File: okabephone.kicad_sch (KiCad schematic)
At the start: 41 parts, among them J1 Micro_SD_Card_Det1, J2 USB_C_Receptacle_USB2.0_16P, M1 Motor_DC, Q1 AO3400A, SW1 SW_Push, SW10 SW_Push, SW11 SW_Push, SW12 SW_Push, SW13 SW_Push, SW14 SW_Push, SW15 SW_Push, SW16 SW_Push, SW17 SW_Push, SW18 SW_Push, SW19 SW_Push, SW2 SW_Push, SW3 SW_Push, SW4 SW_Push, SW5 SW_Push, SW6 SW_Push, SW7 SW_Push, SW8 SW_Push, SW9 SW_Push, U1 MCP23017_ML, U2 ESP32-S3-WROOM-1, U4 SIM7080G, U5 LD1117S33TR_SOT223

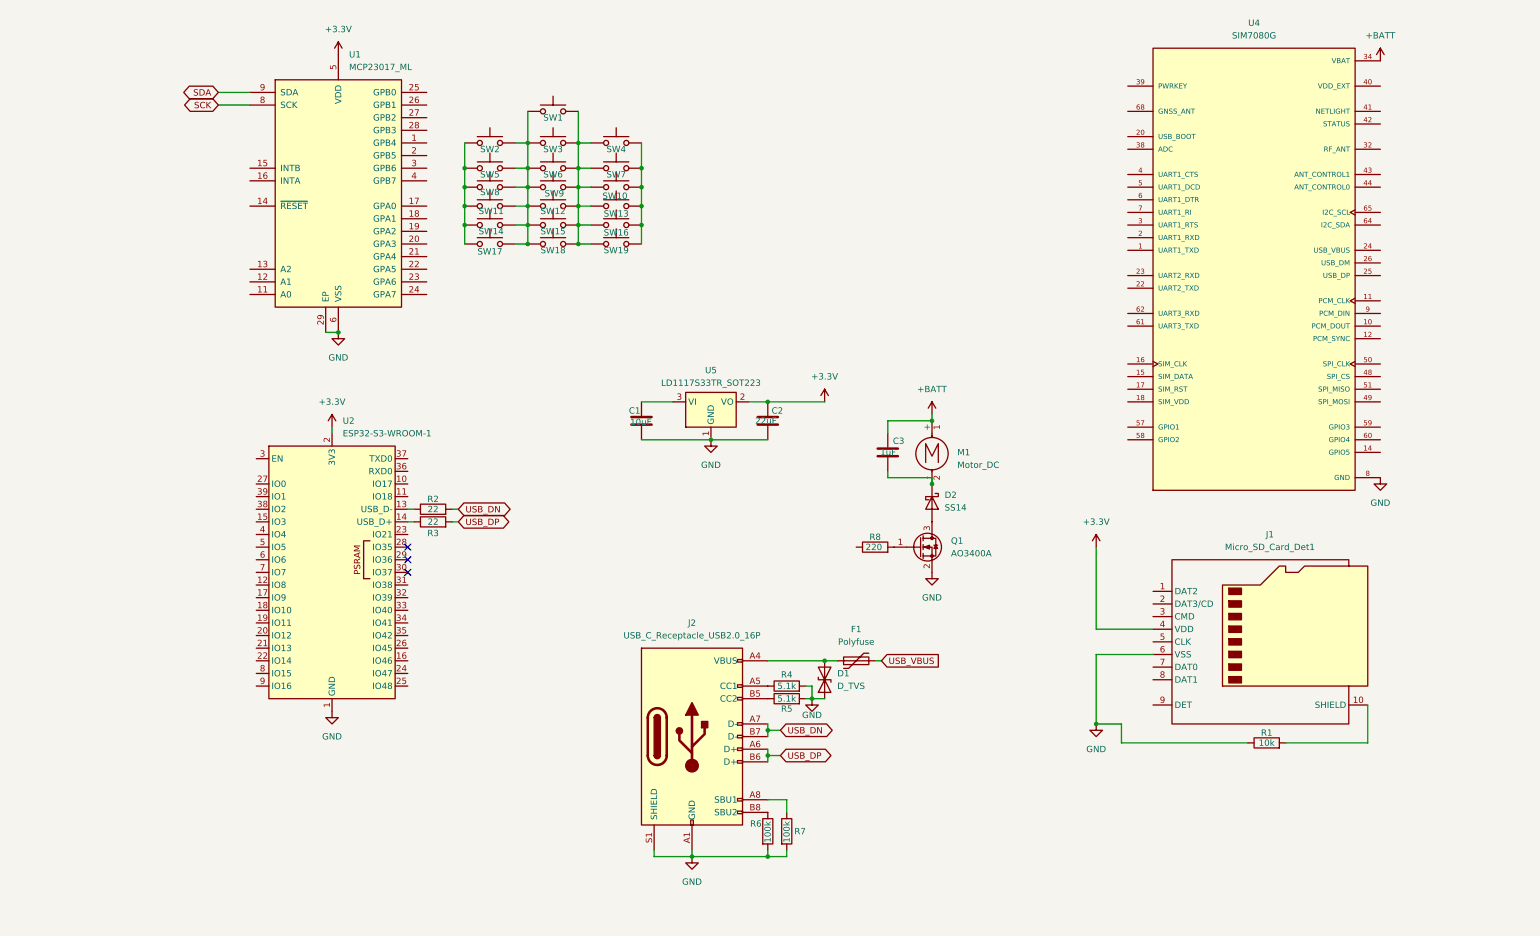
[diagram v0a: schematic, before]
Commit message: SD card and stuff?
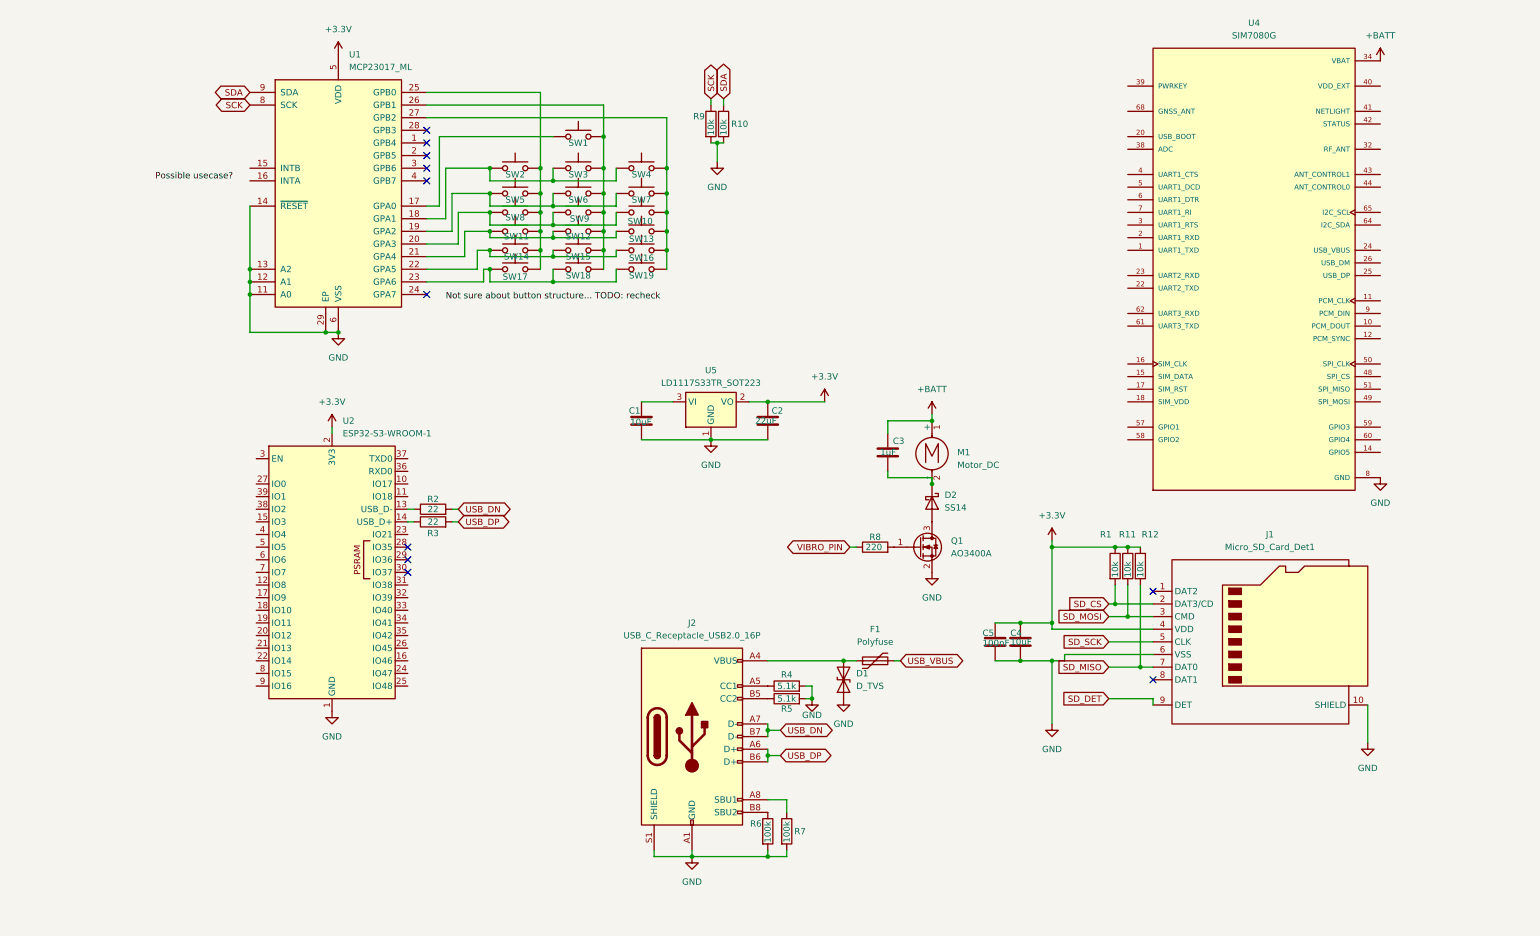
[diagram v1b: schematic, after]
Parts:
- added C4: 10uF, symbol Device:C
- added C5: 100nF, symbol Device:C
- added R10, R11, R12, R9: 10k, symbol Device:R
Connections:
- net +3.3V: now also R1.1, C4.1, C5.1, R11.1, R12.1
- net GND: now also J1.10 (SHIELD), U1.11 (A0), U1.12 (A1), U1.13 (A2), U1.14 (~{RESET}), C4.2, C5.2, R10.2, R9.2; no longer R1.1
- net SCK: now also R9.1
- net SDA: now also R10.1
- net at SW1.2, SW12.2, SW15.2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: now also U1.26 (GPB1); no longer SW10.1, SW13.1, SW16.1, SW19.1, SW4.1, SW7.1
- net at SW10.2, SW13.2, SW16.2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: now also U1.27 (GPB2)
- net VIBRO_PIN: now reaches R8.1
- net at U1.17 (GPA0): now also SW1.1
- net at U1.18 (GPA1): now also SW2.1, SW3.1, SW4.1
- net at U1.19 (GPA2): now also SW5.1, SW6.1, SW7.1
- net at U1.20 (GPA3): now also SW10.1, SW8.1, SW9.1
- net at U1.21 (GPA4): now also SW11.1, SW12.1, SW13.1
- net at U1.22 (GPA5): now also SW14.1, SW15.1, SW16.1
- net at U1.23 (GPA6): now also SW17.1, SW18.1, SW19.1
- net at U1.25 (GPB0): now also SW11.2, SW14.2, SW17.2, SW2.2, SW5.2, SW8.2
- net SD_CS: now reaches R1.2
- net SD_CS: now also J1.2 (DAT3/CD); no longer J1.10 (SHIELD)
- net SD_MOSI: now reaches J1.3 (CMD)
- net SD_MOSI: now also R11.2
- net SD_SCK: now reaches J1.5 (CLK)
- net SD_MISO: now reaches J1.7 (DAT0)
- net SD_MISO: now also R12.2
- net SD_DET: now reaches J1.9 (DET)
- no-connect marks 3 -> 11
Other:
- moved on the sheet: D1, F1, SW1, SW10, SW11, SW12, SW13, SW14, SW15, SW16, SW17, SW18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

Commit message: t
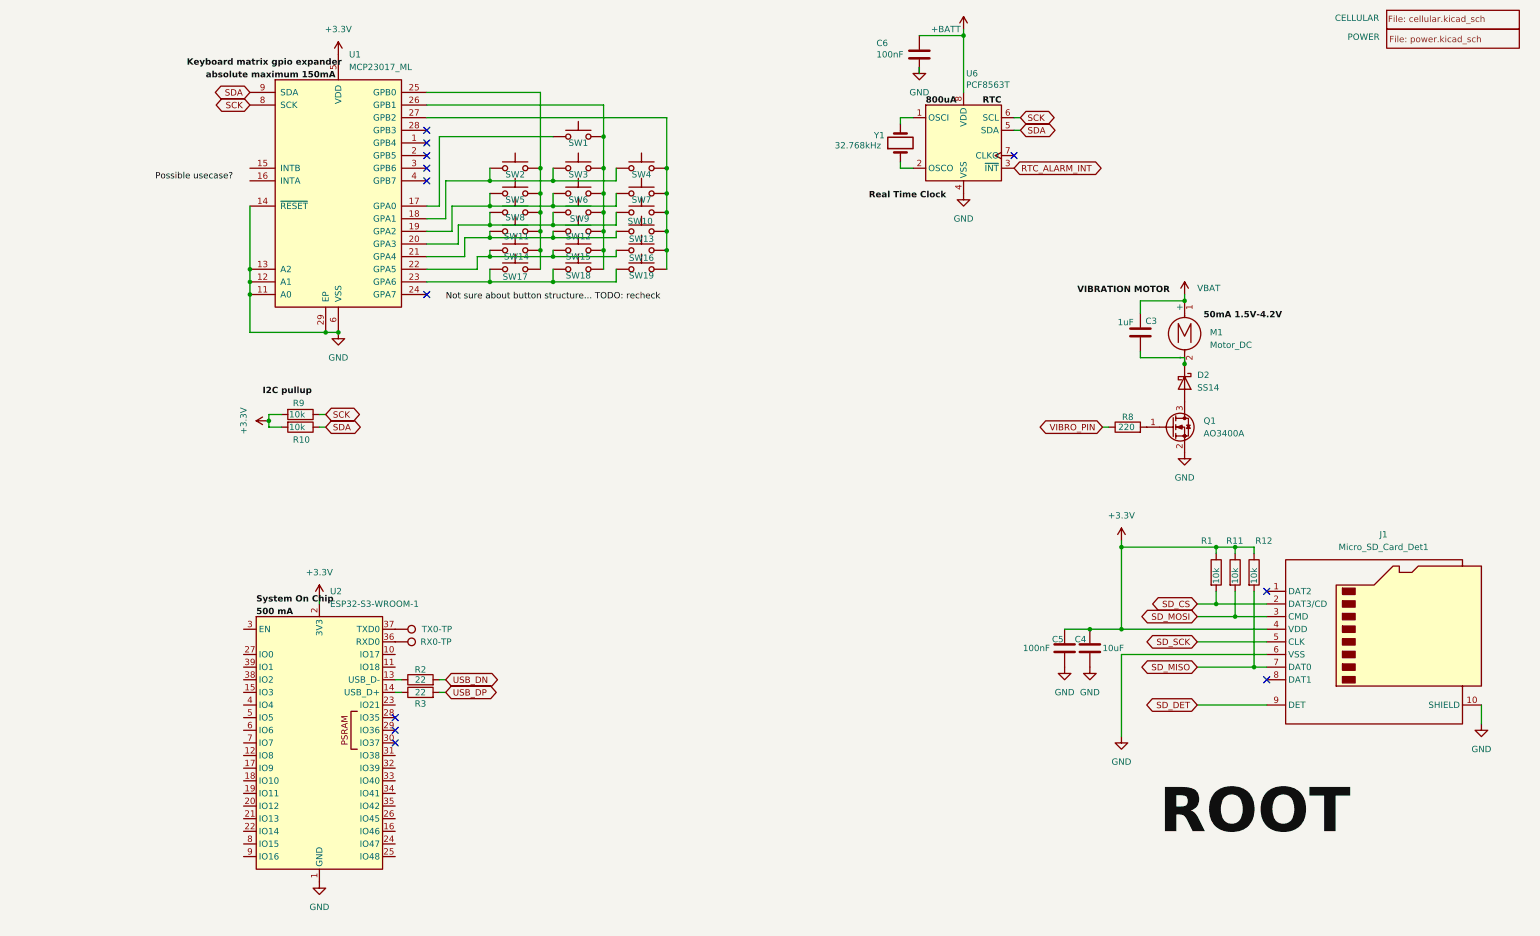
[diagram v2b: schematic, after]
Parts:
- removed C1: 10uF, symbol Device:C
- removed C2: 22uF, symbol Device:C
- removed D1: D_TVS, symbol Device:D_TVS
- removed F1: Polyfuse, symbol Device:Polyfuse
- removed J2: USB_C_Receptacle_USB2.0_16P, symbol Connector:USB_C_Receptacle_USB2.0_16P
- removed R4, R5: 5.1k, symbol Device:R
- removed R6, R7: 100k, symbol Device:R
- removed U4: SIM7080G, SIM7080G:XCVR_SIM7080G, symbol SIM7080G:SIM7080G
- removed U5: LD1117S33TR_SOT223, Package_TO_SOT_SMD:SOT-223-3_TabPin2, symbol Regulator_Linear:LD1117S33TR_SOT223
- added C6: 100nF, symbol Device:C
- added RX0-TP, TX0-TP: TestPoint, symbol Connector:TestPoint
- added U6: PCF8563T, Package_SO:SOIC-8_3.9x4.9mm_P1.27mm, symbol Timer_RTC:PCF8563T
- added Y1: 32.768kHz, Crystal:Crystal_SMD_3215-2Pin_3.2x1.5mm, symbol Device:Crystal
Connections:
- net +3.3V: now also R10.2, R9.2
- net +BATT: now also C6.1, U6.8 (VDD); no longer C3.1, M1.1 (+)
- net GND: now also C6.2, U6.4 (VSS); no longer R10.2, R9.2
- net SCK: now also U6.6 (SCL)
- net SDA: now also U6.5 (SDA)
- net at U2.36 (RXD0): now also RX0-TP.1
- net at U2.37 (TXD0): now also TX0-TP.1
- new net: U6.1 (OSCI), Y1.2
- new net: U6.2 (OSCO), Y1.1
- new net RTC_ALARM_INT: U6.3 (~{INT})
- new net VBAT: C3.1, M1.1 (+)
- no-connect marks 11 -> 12
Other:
- added sheet CELLULAR (cellular.kicad_sch)
- added sheet POWER (power.kicad_sch)
- company: (none) -> Nergon
- title: (none) -> Okabe_Phone
- moved on the sheet: C3, C4, C5, D2, J1, M1, Q1, R1, R10, R11, R12, R2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

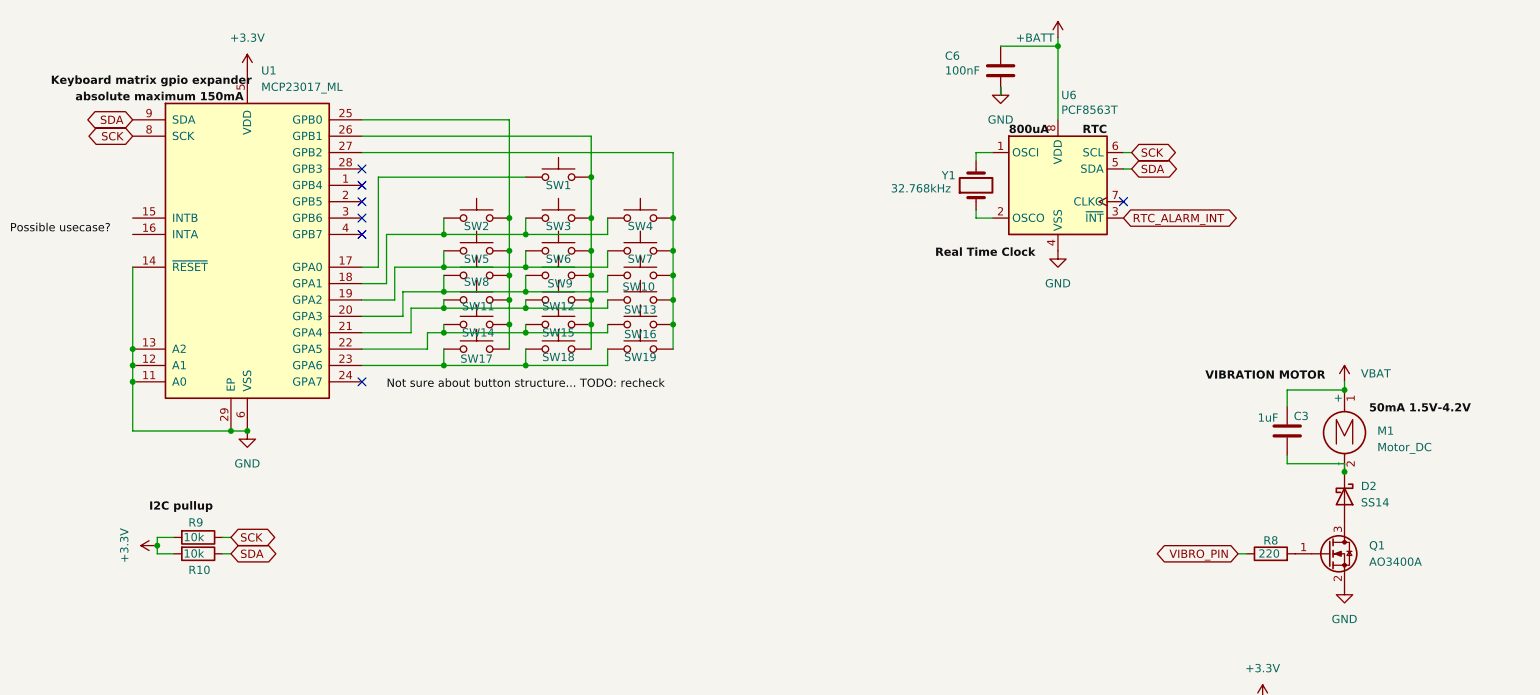
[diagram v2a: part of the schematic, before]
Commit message: power
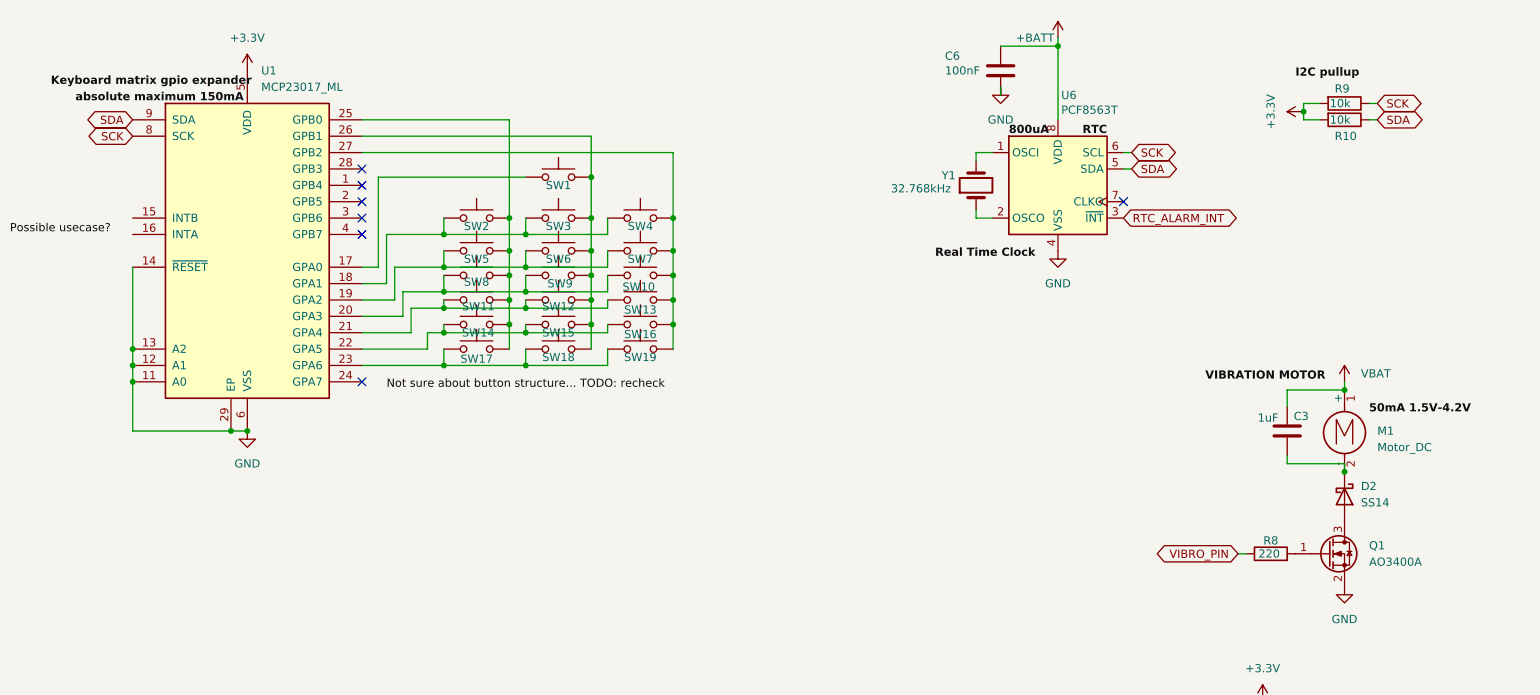
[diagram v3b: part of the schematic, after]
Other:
- moved on the sheet: R10, R9
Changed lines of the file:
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@@
 	)
 	(junction
-		(at 33.02 95.25)
+		(at 210.82 27.94)
 		(diameter 0)
 		(color 0 0 0 0)
@@
 	(wire
 		(pts
-			(xy 33.02 93.98) (xy 35.56 93.98)
+			(xy 210.82 26.67) (xy 213.36 26.67)
 		)
 		(stroke
@@
 	(wire
 		(pts
-			(xy 44.45 93.98) (xy 43.18 93.98)
+			(xy 222.25 26.67) (xy 220.98 26.67)
 		)
 		(stroke
@@
 	(wire
 		(pts
-			(xy 44.45 96.52) (xy 43.18 96.52)
+			(xy 222.25 29.21) (xy 220.98 29.21)
 		)
 		(stroke
@@
 	(wire
 		(pts
-			(xy 33.02 93.98) (xy 33.02 95.25)
+			(xy 210.82 26.67) (xy 210.82 27.94)
 		)
 		(stroke
@@
 	(wire
 		(pts
-			(xy 33.02 96.52) (xy 35.56 96.52)
+			(xy 210.82 29.21) (xy 213.36 29.21)
 		)
 		(stroke
@@
 	(wire
 		(pts
-			(xy 33.02 96.52) (xy 33.02 95.25)
+			(xy 210.82 29.21) (xy 210.82 27.94)
 		)
 		(stroke
@@
 	)
 	(label "I2C pullup"
-		(at 31.75 90.17 0)
+		(at 209.55 22.86 0)
 		(effects
 			(font
@@
 	(global_label "SDA"
 		(shape bidirectional)
-		(at 44.45 96.52 0)
+		(at 222.25 29.21 0)
 		(fields_autoplaced yes)
 		(effects
@@
 		)
 		(property "Intersheetrefs" "${INTERSHEET_REFS}"
-			(at 52.1146 96.52 0)
+			(at 229.9146 29.21 0)
 			(effects
 				(font
@@
 	(global_label "SCK"
 		(shape bidirectional)
-		(at 44.45 93.98 0)
+		(at 222.25 26.67 0)
 		(fields_autoplaced yes)
 		(effects
@@
 		)
 		(property "Intersheetrefs" "${INTERSHEET_REFS}"
-			(at 52.296 93.98 0)
+			(at 230.096 26.67 0)
 			(effects
 				(font
@@
 	(symbol
 		(lib_id "Device:R")
-		(at 39.37 93.98 270)
+		(at 217.17 26.67 270)
 		(unit 1)
 		(exclude_from_sim no)
@@
 		(dnp no)
 		(property "Reference" "R9"
-			(at 37.846 91.694 90)
+			(at 215.646 24.384 90)
 			(effects
 				(font
@@
 		)
 		(property "Value" "10k"
-			(at 37.084 93.98 90)
+			(at 214.884 26.67 90)
 			(effects
 				(font
@@
 		)
 		(property "Footprint" ""
-			(at 39.37 92.202 90)
+			(at 217.17 24.892 90)
 			(effects
 				(font
@@
 		)
 		(property "Datasheet" "~"
-			(at 39.37 93.98 0)
+			(at 217.17 26.67 0)
 			(effects
 				(font
@@
 		)
 		(property "Description" "Resistor"
-			(at 39.37 93.98 0)
+			(at 217.17 26.67 0)
 			(effects
 				(font
@@
 	(symbol
 		(lib_id "power:+3.3V")
-		(at 33.02 95.25 90)
+		(at 210.82 27.94 90)
 		(unit 1)
 		(exclude_from_sim no)
@@
 		(dnp no)
 		(property "Reference" "#PWR06"
-			(at 36.83 95.25 0)
+			(at 214.63 27.94 0)
 			(effects
 				(font
@@
 		)
 		(property "Value" "+3.3V"
-			(at 27.94 95.25 0)
+			(at 205.74 27.94 0)
 			(effects
 				(font
@@
 		)
 		(property "Footprint" ""
-			(at 33.02 95.25 0)
+			(at 210.82 27.94 0)
 			(effects
 				(font
@@
 		)
 		(property "Datasheet" ""
-			(at 33.02 95.25 0)
+			(at 210.82 27.94 0)
 			(effects
 				(font
@@
 		)
 		(property "Description" "Power symbol creates a global label with name \"+3.3V\""
-			(at 33.02 95.25 0)
+			(at 210.82 27.94 0)
 			(effects
 				(font
@@
 		(on_board yes)
 		(dnp no)
-		(fields_autoplaced yes)
 		(property "Reference" "#PWR07"
 			(at 46.99 83.82 0)
@@
 	(symbol
 		(lib_id "Device:R")
-		(at 39.37 96.52 270)
+		(at 217.17 29.21 270)
 		(unit 1)
 		(exclude_from_sim no)
@@
 		(dnp no)
 		(property "Reference" "R10"
-			(at 37.846 99.06 90)
+			(at 215.646 31.75 90)
 			(effects
 				(font
@@
 		)
 		(property "Value" "10k"
-			(at 37.084 96.52 90)
+			(at 214.884 29.21 90)
 			(effects
 				(font
@@
 		)
 		(property "Footprint" ""
-			(at 39.37 94.742 90)
+			(at 217.17 27.432 90)
 			(effects
 				(font
@@
 		)
 		(property "Datasheet" "~"
-			(at 39.37 96.52 0)
+			(at 217.17 29.21 0)
 			(effects
 				(font
@@
 		)
 		(property "Description" "Resistor"
-			(at 39.37 96.52 0)
+			(at 217.17 29.21 0)
 			(effects
 				(font
